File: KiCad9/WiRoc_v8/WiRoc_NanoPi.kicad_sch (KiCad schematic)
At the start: 49 parts, among them J1 Conn_02x05_Odd_Even, J10 Conn_01x09_Socket, J2 Conn_01x04, J5 Conn_01x04_Socket, J6 HAT_Conn_DBG, J8 Conn_01x06, SW1 SW_SPST, U2 OLED, U3 AXP209, U5 SY6280, U6 BatteryPadM, U7 BatteryPadP

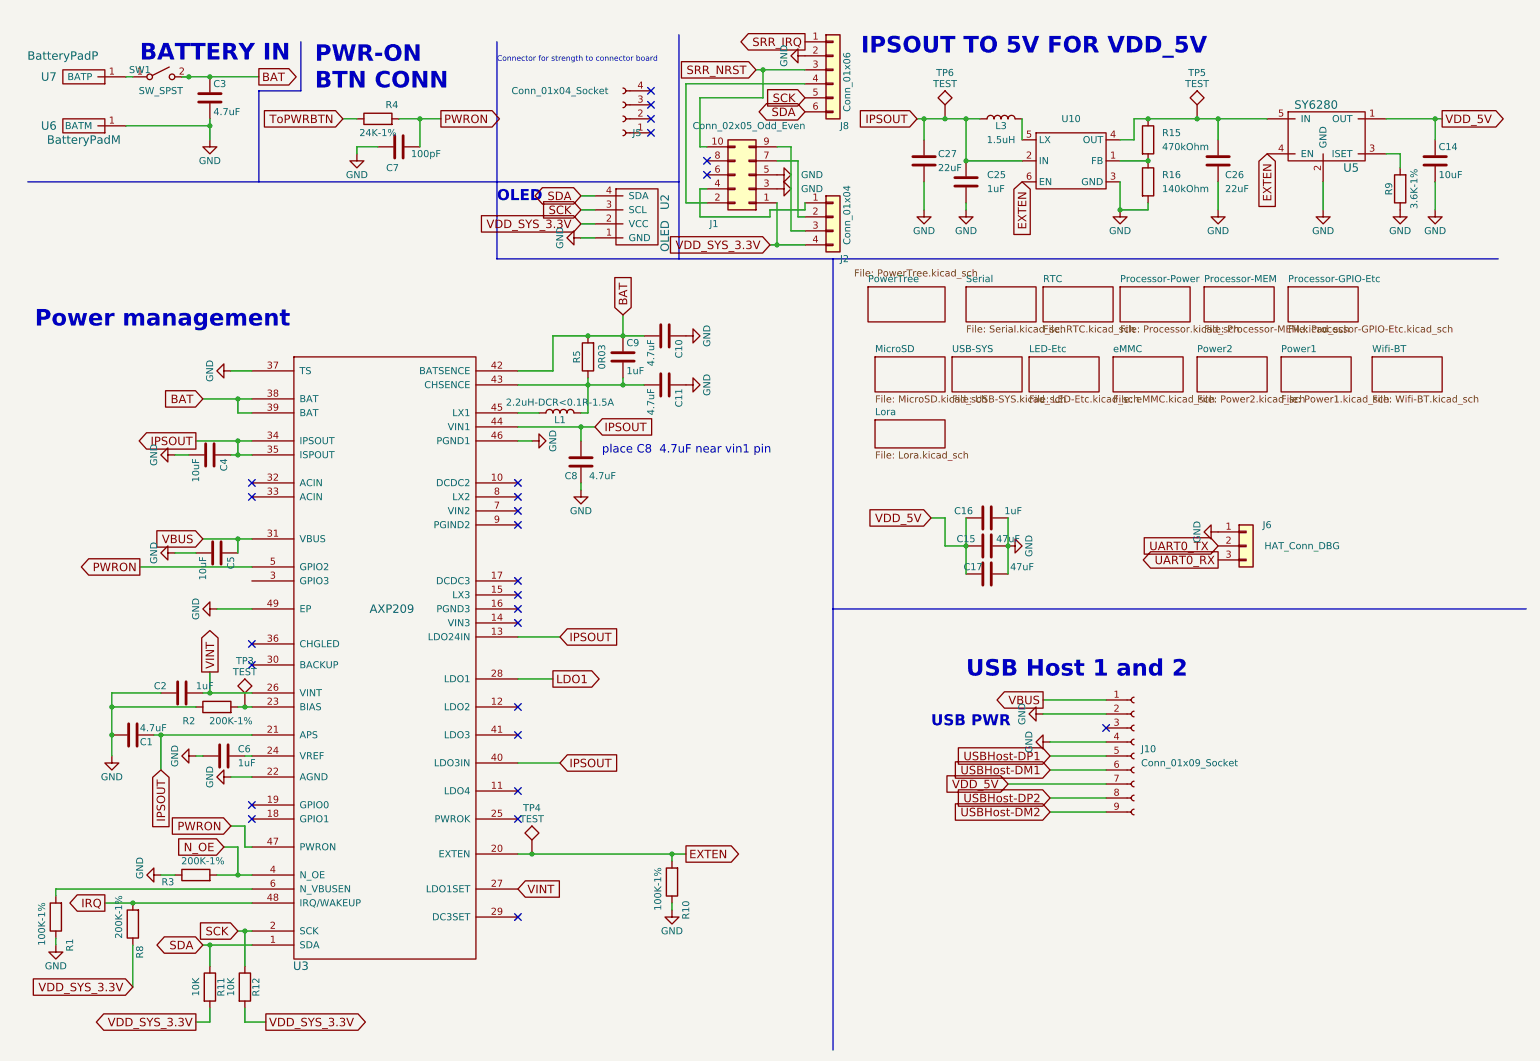
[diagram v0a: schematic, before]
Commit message: etc
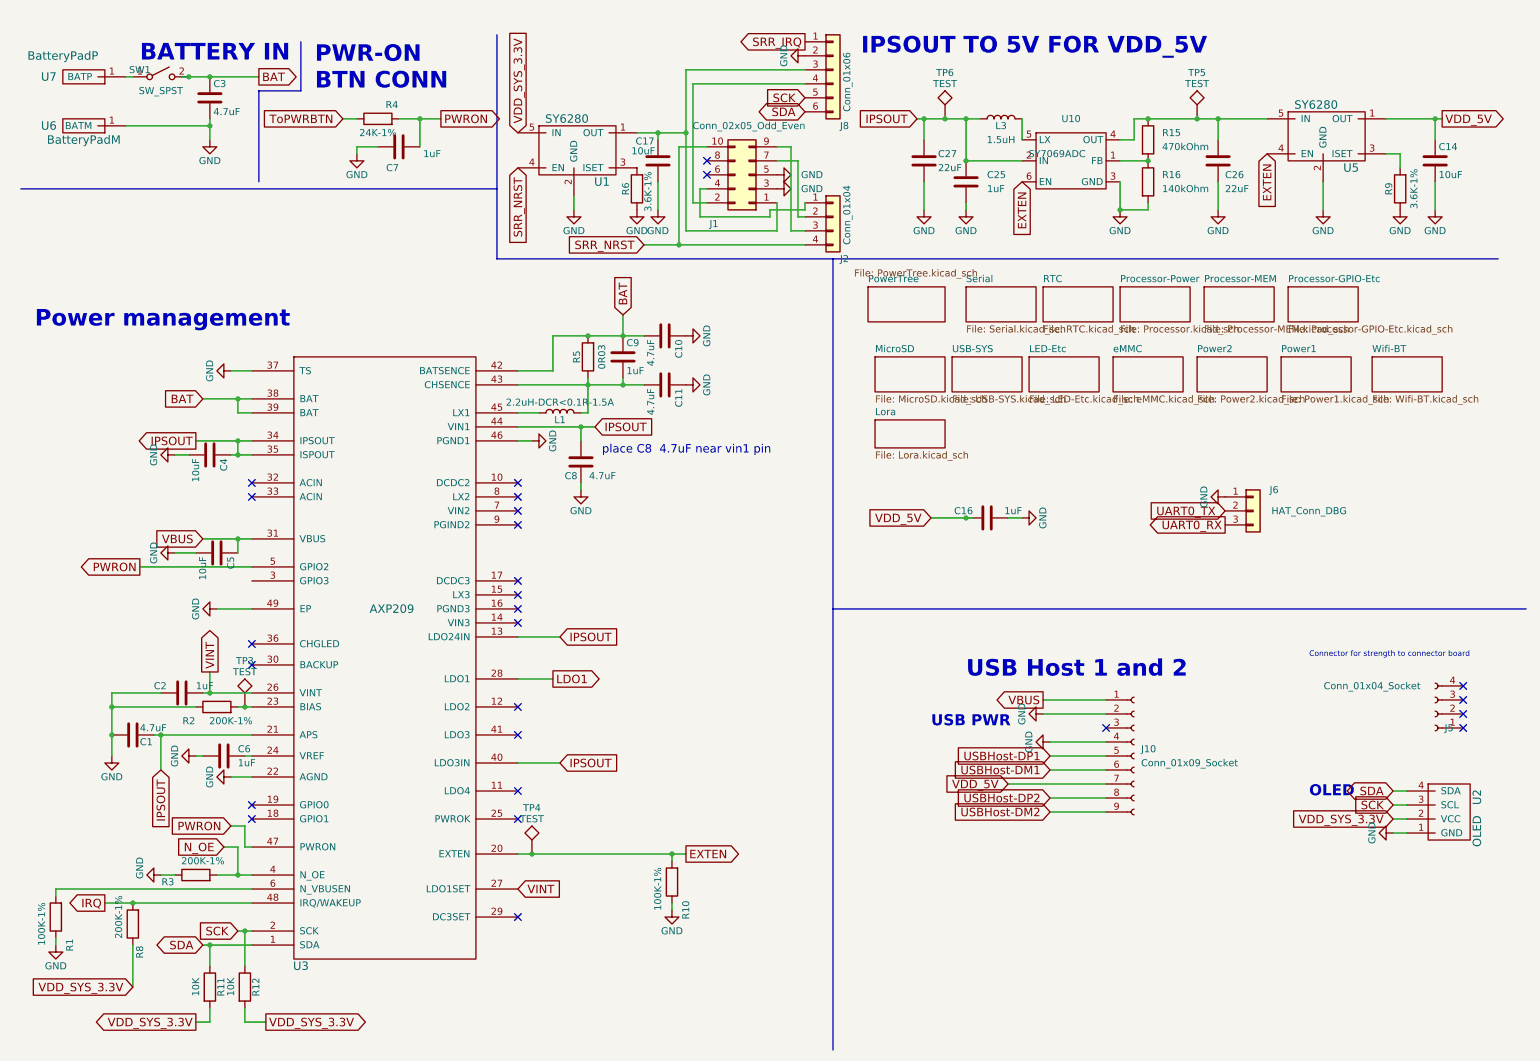
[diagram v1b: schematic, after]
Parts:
- removed C15: 47uF, Capacitor_SMD:C_1206_3216Metric, symbol Device:C
- added R6: 3.6K-1%, Resistor_SMD:R_0402_1005Metric, symbol Device:R
- added U1: SY6280, Package_TO_SOT_SMD:SOT-23-5, symbol WiRoc:SY6280
- C1, C10, C11, C3, C8: LCSC Part # C19666 -> C23733; ManufacturerPartNumber CL10A475KO8NNNC -> CL05A475MP5NRNC
- C14, C4, C5: LCSC Part # C19702 -> C15525; ManufacturerPartNumber CL10A106KP8NNNC -> CL05A106MQ5NUNC
- C16, C2, C25, C6, C9: LCSC Part # C15849 -> C52923; ManufacturerPartNumber CL10A105KB8NNNC -> CL05A105KA5NQNC
- C17: value 47uF -> 10uF; footprint Capacitor_SMD:C_1206_3216Metric -> Capacitor_SMD:C_0402_1005Metric; LCSC Part # C96123 -> C15525; Manufacturer Murata Electronics -> Samsung Electro-Mechanics; ManufacturerPartNumber CL31A476MPHNNNE -> CL05A106MQ5NUNC; Package 1206 -> 0603; WebsiteURL (none) -> https://lcsc.com/product-detail/Multilayer-Ceramic-Capacito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
- C26, C27: footprint Capacitor_SMD:C_0402_1005Metric -> Capacitor_SMD:C_0603_1608Metric
- C7: value 100pF -> 1uF; LCSC Part # C14858 -> C52923; ManufacturerPartNumber CL10C101JB8NNNC -> CL05A105KA5NQNC
- U10: value ~ -> SY7069ADC
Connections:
- net GND: now also C17.2, R6.1, U1.2 (GND); no longer C17.1
- net SRR_NRST: now also J2.4 (Pin_4), U1.4 (EN); no longer J8.3 (Pin_3)
- net VDD_5V: no longer C17.2
- net VDD_SYS_3.3V: now also U1.5 (IN); no longer J1.1 (Pin_1), J2.4 (Pin_4)
- new net: R6.2, U1.3 (ISET)
- new net: C17.1, J1.1 (Pin_1), J8.3 (Pin_3), U1.1 (OUT)
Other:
- moved on the sheet: J5, J6, U2
